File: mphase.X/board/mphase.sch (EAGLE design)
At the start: 36 parts, among them IC1 MAX232, IC2 PIC18F4455_40, X1 332-10, X2 332-10

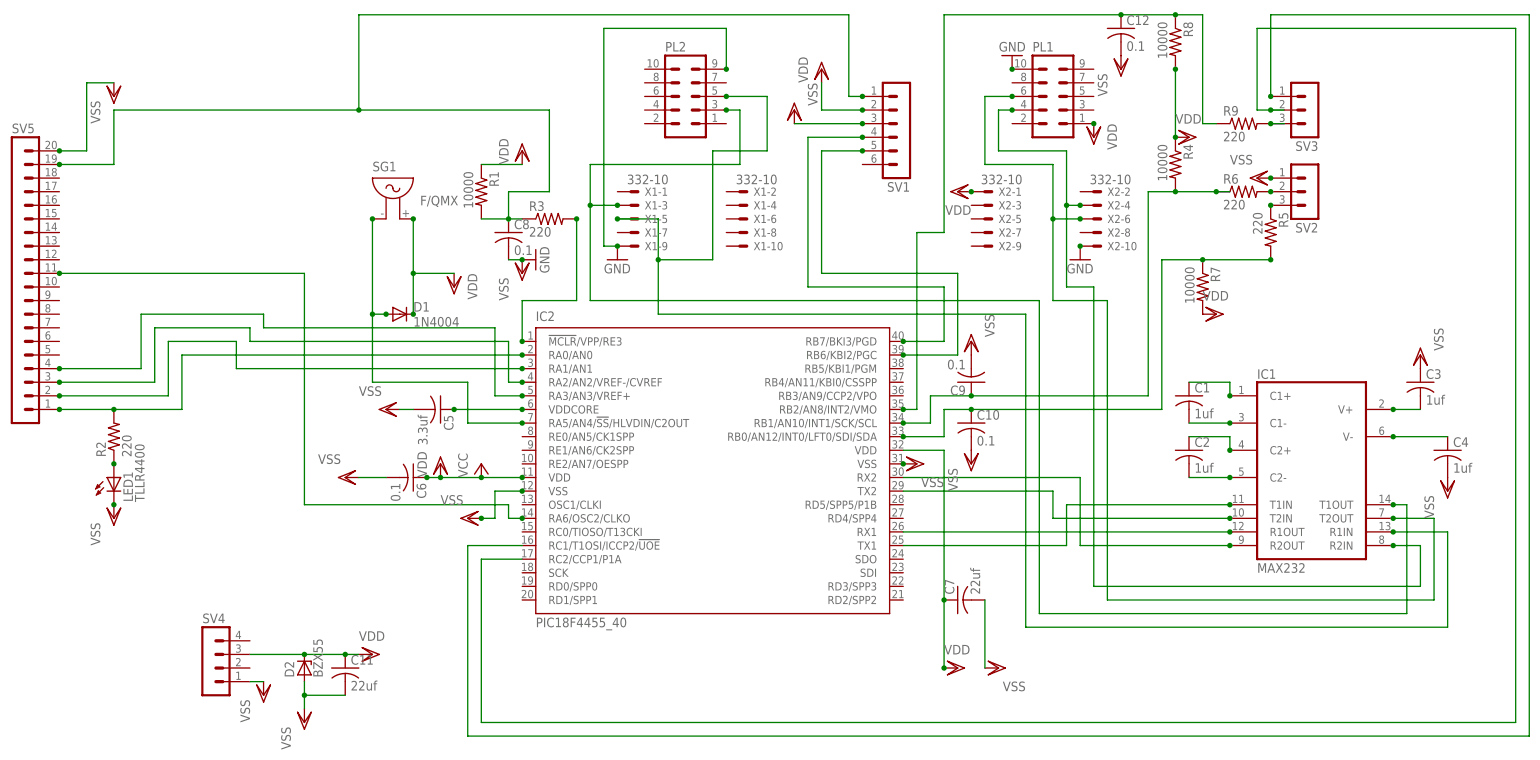
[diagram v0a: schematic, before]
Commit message: up
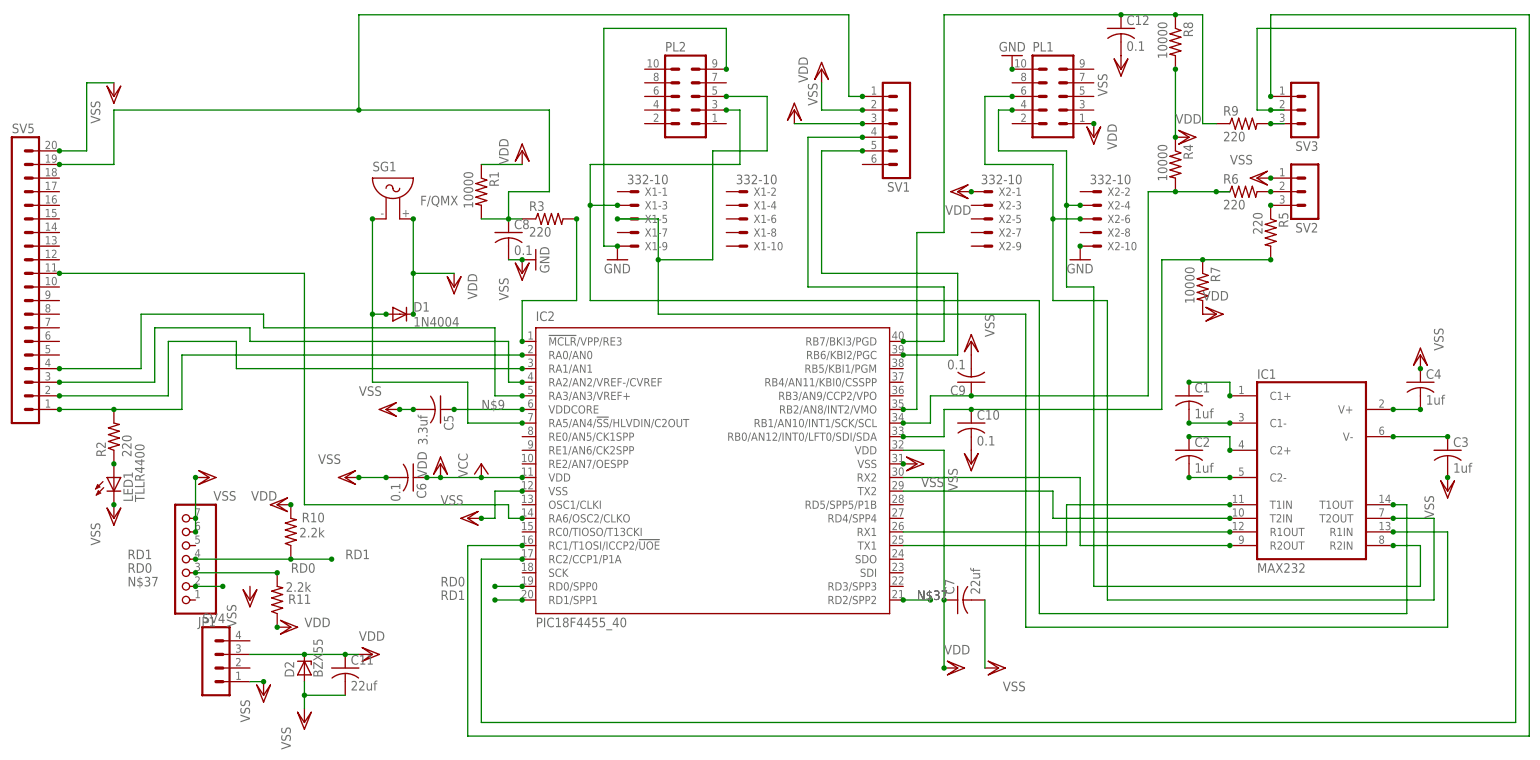
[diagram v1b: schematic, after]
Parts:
- added JP1: (no value), pinhead:PINHD-1X7
- added R10, R11: 2.2k, resistor:R-US_0204/2V
- C1, C2, C3, C4: device resistor:C-US025-025X050 -> rcl:C-USC1206
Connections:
- new net N$37: IC2.RD2/SPP2, JP1.2
- new net RD0: IC2.RD0/SPP0, JP1.3, R11.2
- new net RD1: IC2.RD1/SPP1, JP1.4, R10.1
- net N$5: now also C4.2; no longer C3.2
- net N$6: now also C3.1; no longer C4.1
- net VDD: now also R10.2, R11.1
- net VSS: now also C3.2, C4.1, JP1.6, JP1.7; no longer C3.1, C4.2
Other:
- moved on the sheet: C3, C4
